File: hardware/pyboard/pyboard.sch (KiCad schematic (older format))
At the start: 42 parts

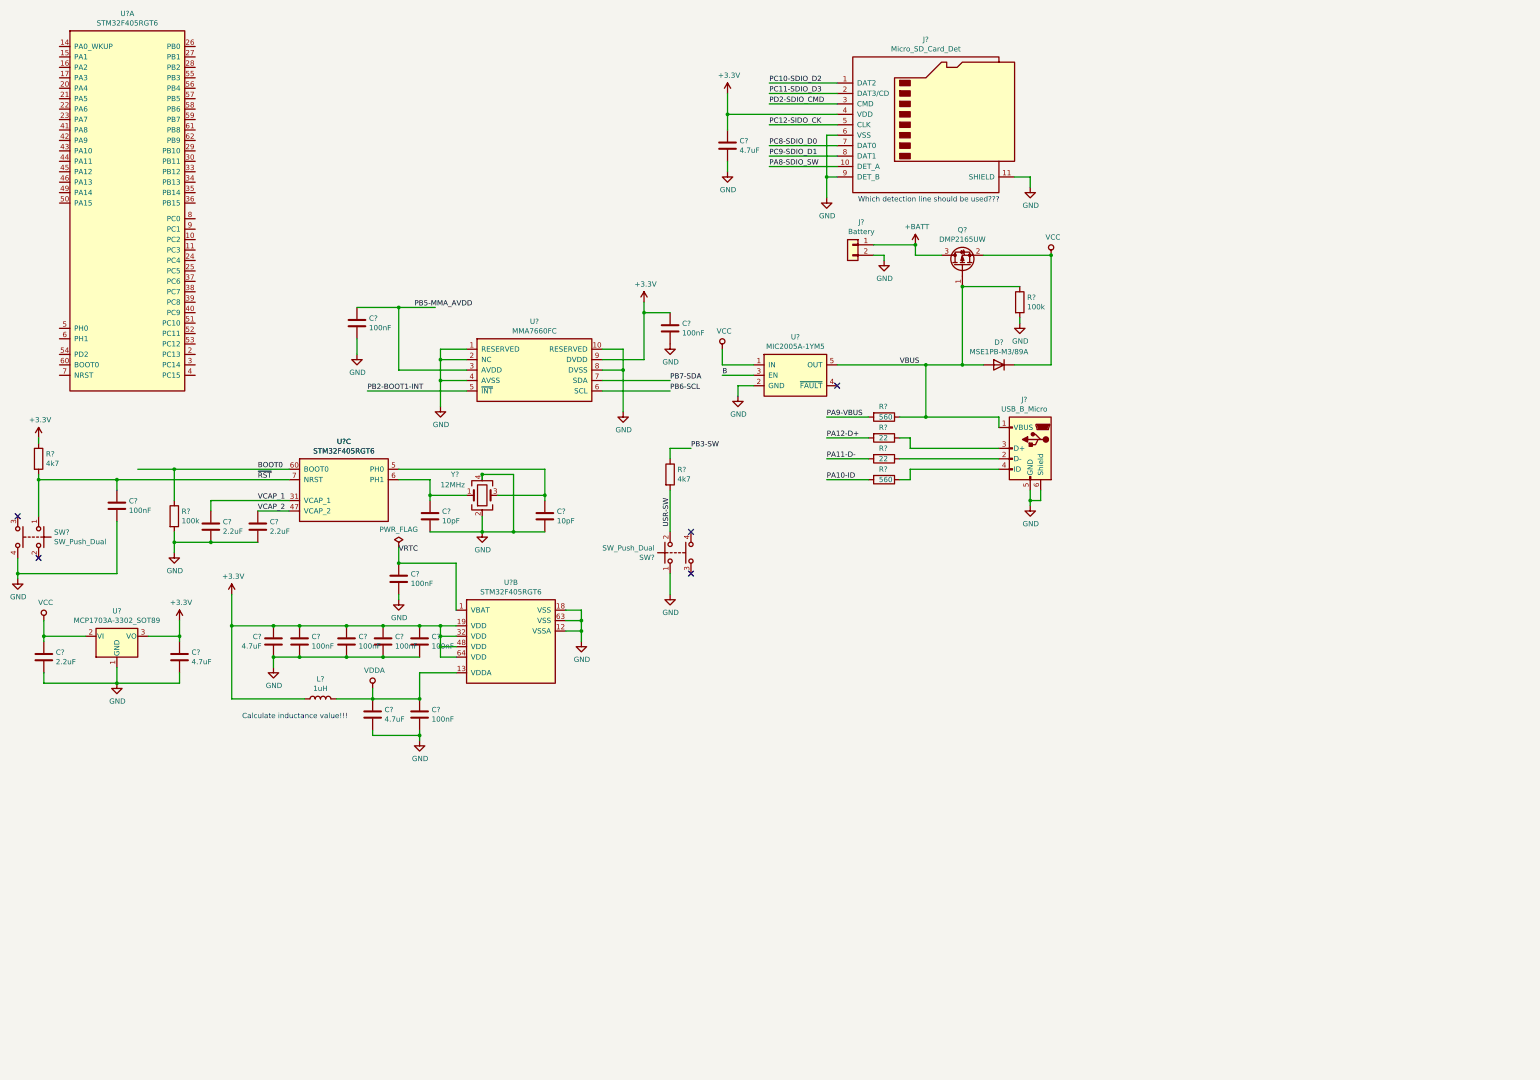
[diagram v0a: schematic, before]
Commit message: Add ports
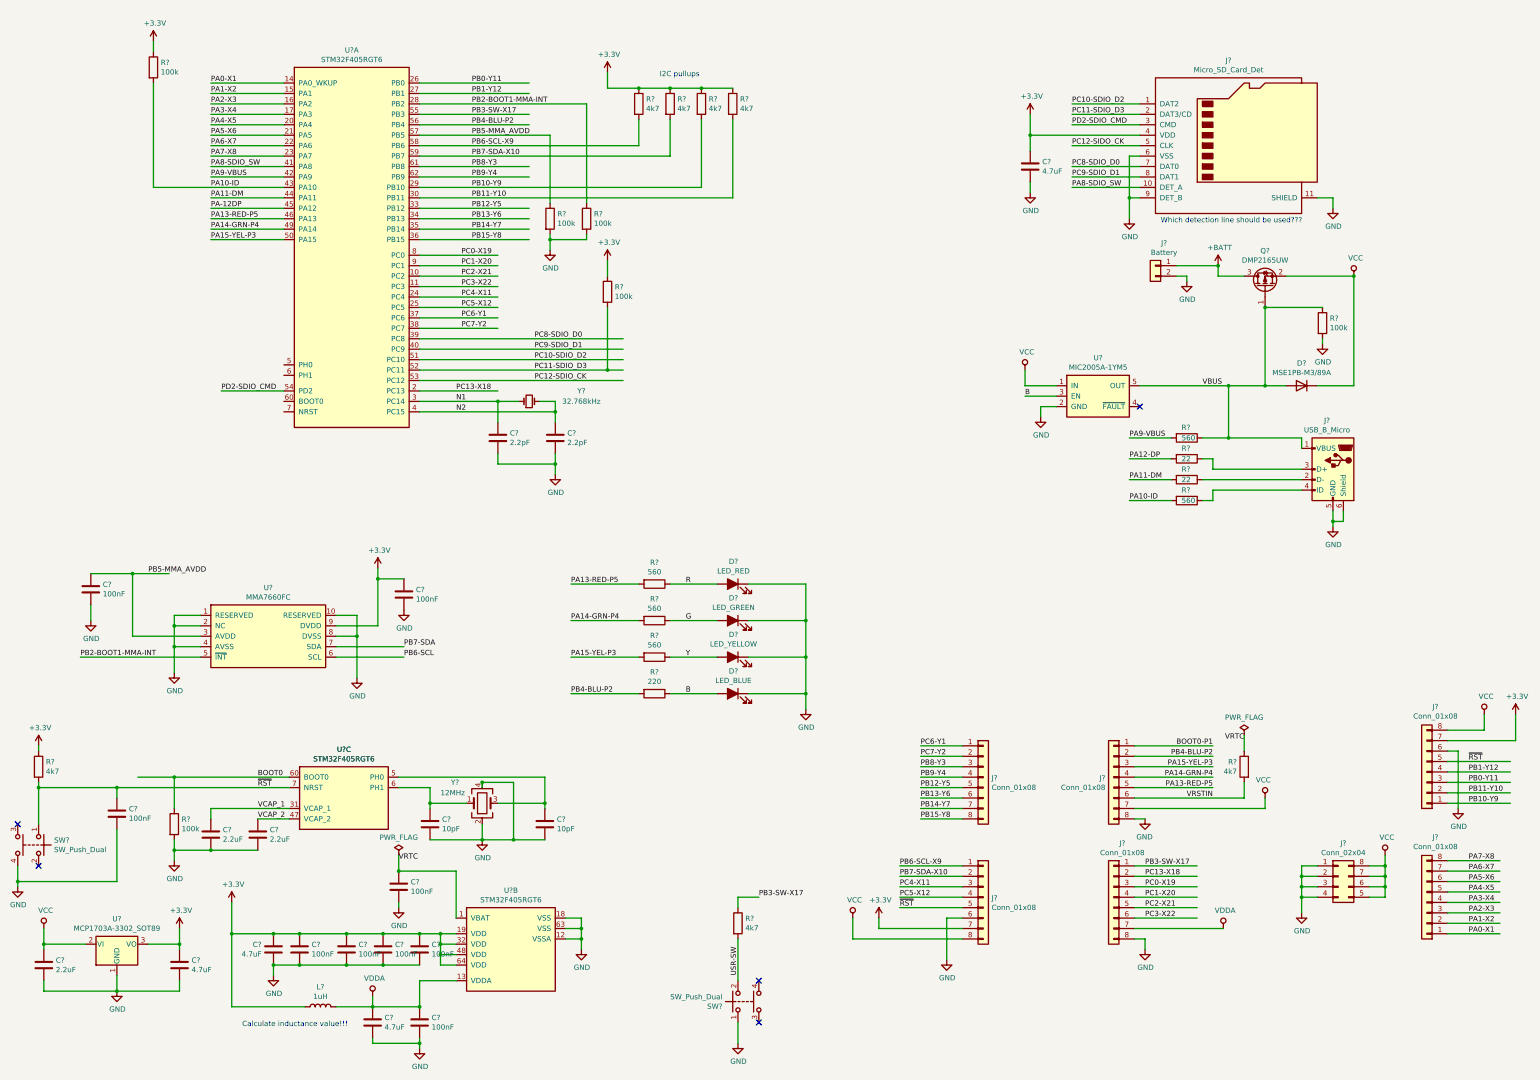
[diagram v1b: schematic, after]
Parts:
- added C? (x2): 2.2pF, symbol Device:C
- added D?: LED_RED, symbol Device:LED_ALT
- added D?: LED_GREEN, symbol Device:LED_ALT
- added D?: LED_YELLOW, symbol Device:LED_ALT
- added D?: LED_BLUE, symbol Device:LED_ALT
- added J? (x6): Conn_01x08, symbol Connector_Generic:Conn_01x08
- added J?: Conn_02x04, symbol Connector_Generic:Conn_02x04_Counter_Clockwise
- added R? (x3): 560, symbol Device:R
- added R?: 220, symbol Device:R
- added R? (x5): 4k7, symbol Device:R
- added R? (x4): 100k, symbol Device:R
- added Y?: 32.768kHz, symbol Device:Crystal_Small
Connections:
- net labels added: BOOT0-P1, G, N1, N2, PA-12DP, PA0-X1, PA1-X2, PA11-DM, PA12-DP, PA13-RED-P5, PA14-GRN-P4, PA15-YEL-P3, PA2-X3, PA3-X4, PA4-X5, PA5-X6, PA6-X7, PA7-X8, PB0-Y11, PB1-Y12, PB10-Y9, PB11-Y10, PB12-Y5, PB13-Y6, PB14-Y7, PB15-Y8, PB2-BOOT1-MMA-INT, PB3-SW-X17, PB4-BLU-P2, PB6-SCL-X9, PB7-SDA-X10, PB8-Y3, PB9-Y4, PC0-X19, PC1-X20, PC12-SDIO_CK, PC13-X18, PC2-X21, PC3-X22, PC4-X11, PC5-X12, PC6-Y1, PC7-Y2, R, VRSTIN, Y
- net labels removed: PA11-D-, PA12-D+, PB2-BOOT1-INT, PB3-SW
- wire segments 167 -> 335
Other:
- note added: "I2C pullups\n"
- moved on the sheet: C?, D?, J?, L?, Q?, R?, SW?, U?, U?A, U?B, U?C, Y?
